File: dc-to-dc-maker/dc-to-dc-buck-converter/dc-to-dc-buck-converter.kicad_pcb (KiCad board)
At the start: 2 copper layers, 1 part, among them U1 IRF640NPBF

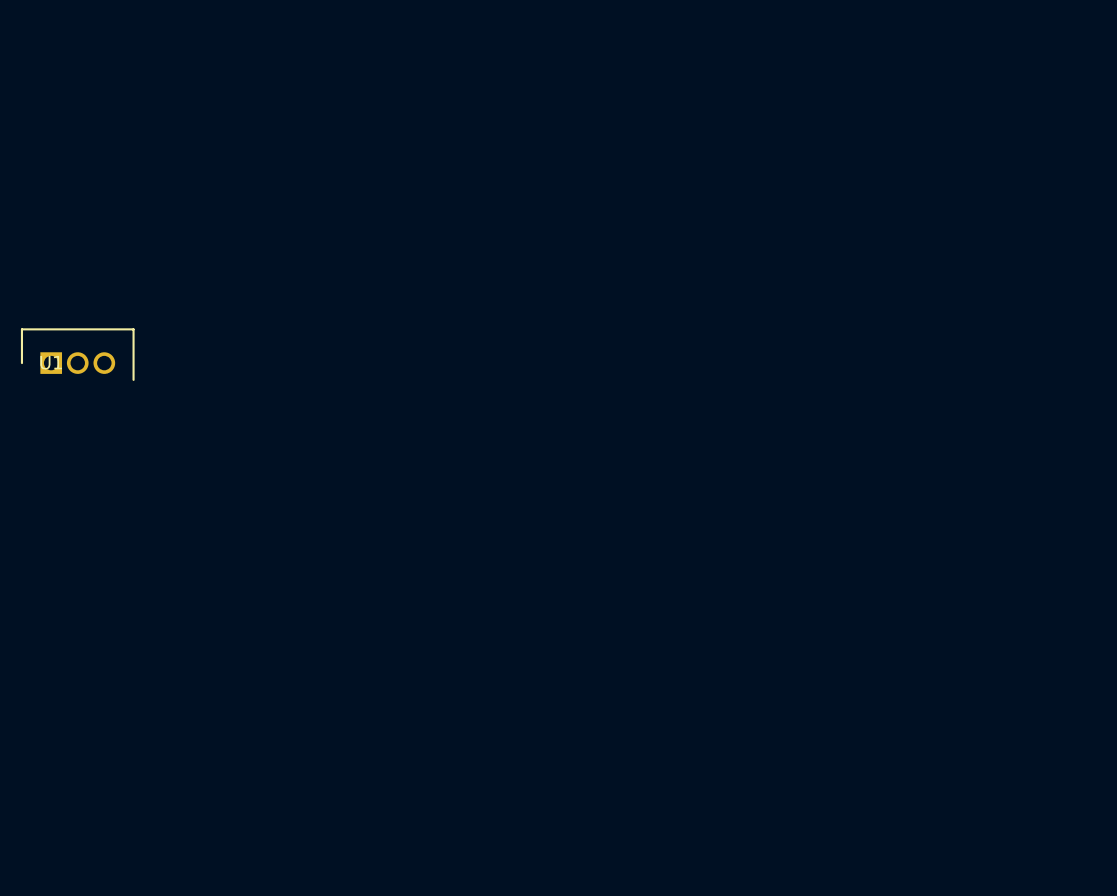
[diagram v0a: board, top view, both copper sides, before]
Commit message: pcb structure + images
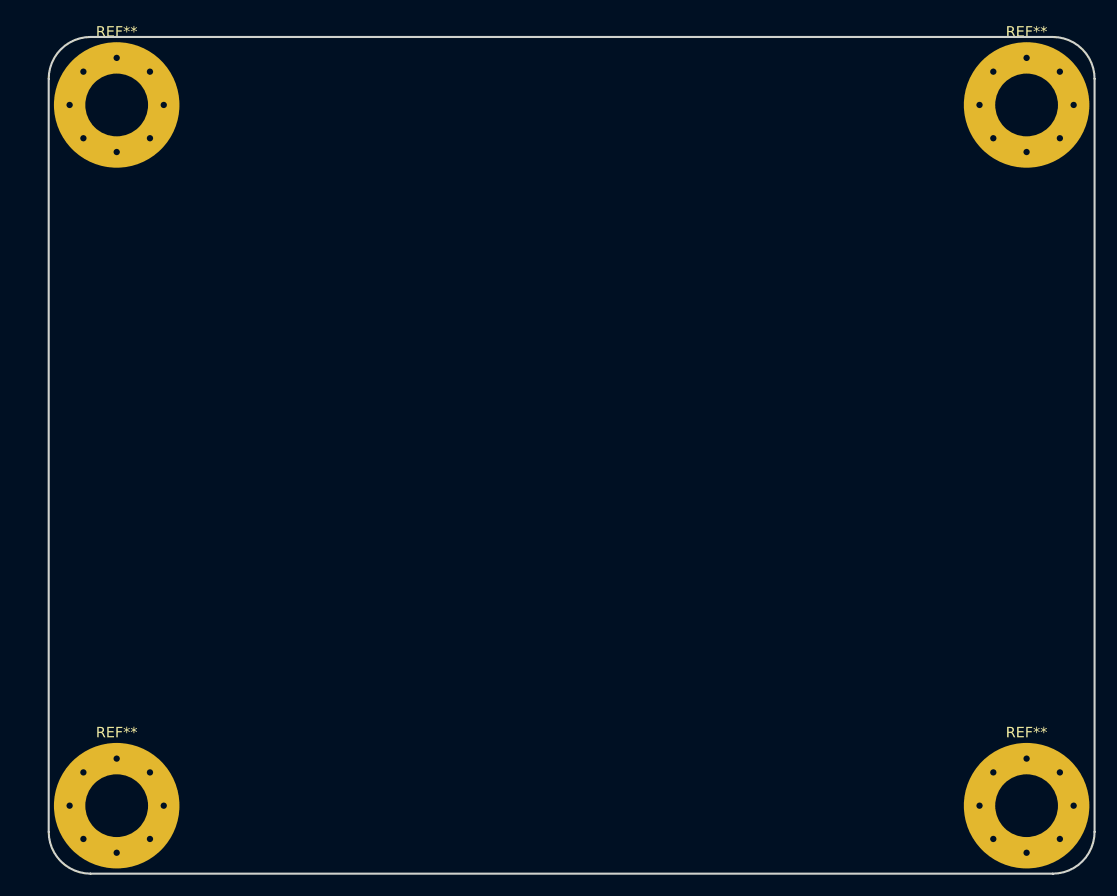
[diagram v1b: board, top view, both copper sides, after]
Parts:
- removed U1: IRF640NPBF, IRF640NPBF:TO254P483X1016X1994-3P
- added REF**: MountingHole_6mm_Pad_Via, MountingHole:MountingHole_6mm_Pad_Via, F.Cu at (191.7, 65.3)
- added REF**: MountingHole_6mm_Pad_Via, MountingHole:MountingHole_6mm_Pad_Via, F.Cu at (104.7, 65.3)
- added REF**: MountingHole_6mm_Pad_Via, MountingHole:MountingHole_6mm_Pad_Via, F.Cu at (191.7, 132.3)
- added REF**: MountingHole_6mm_Pad_Via, MountingHole:MountingHole_6mm_Pad_Via, F.Cu at (104.7, 132.3)
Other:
- board outline added: 100 x 80 mm
